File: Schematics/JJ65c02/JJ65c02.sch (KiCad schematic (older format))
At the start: 22 parts, among them U1 74HC00, U2 74HC02, X1 1Mhz

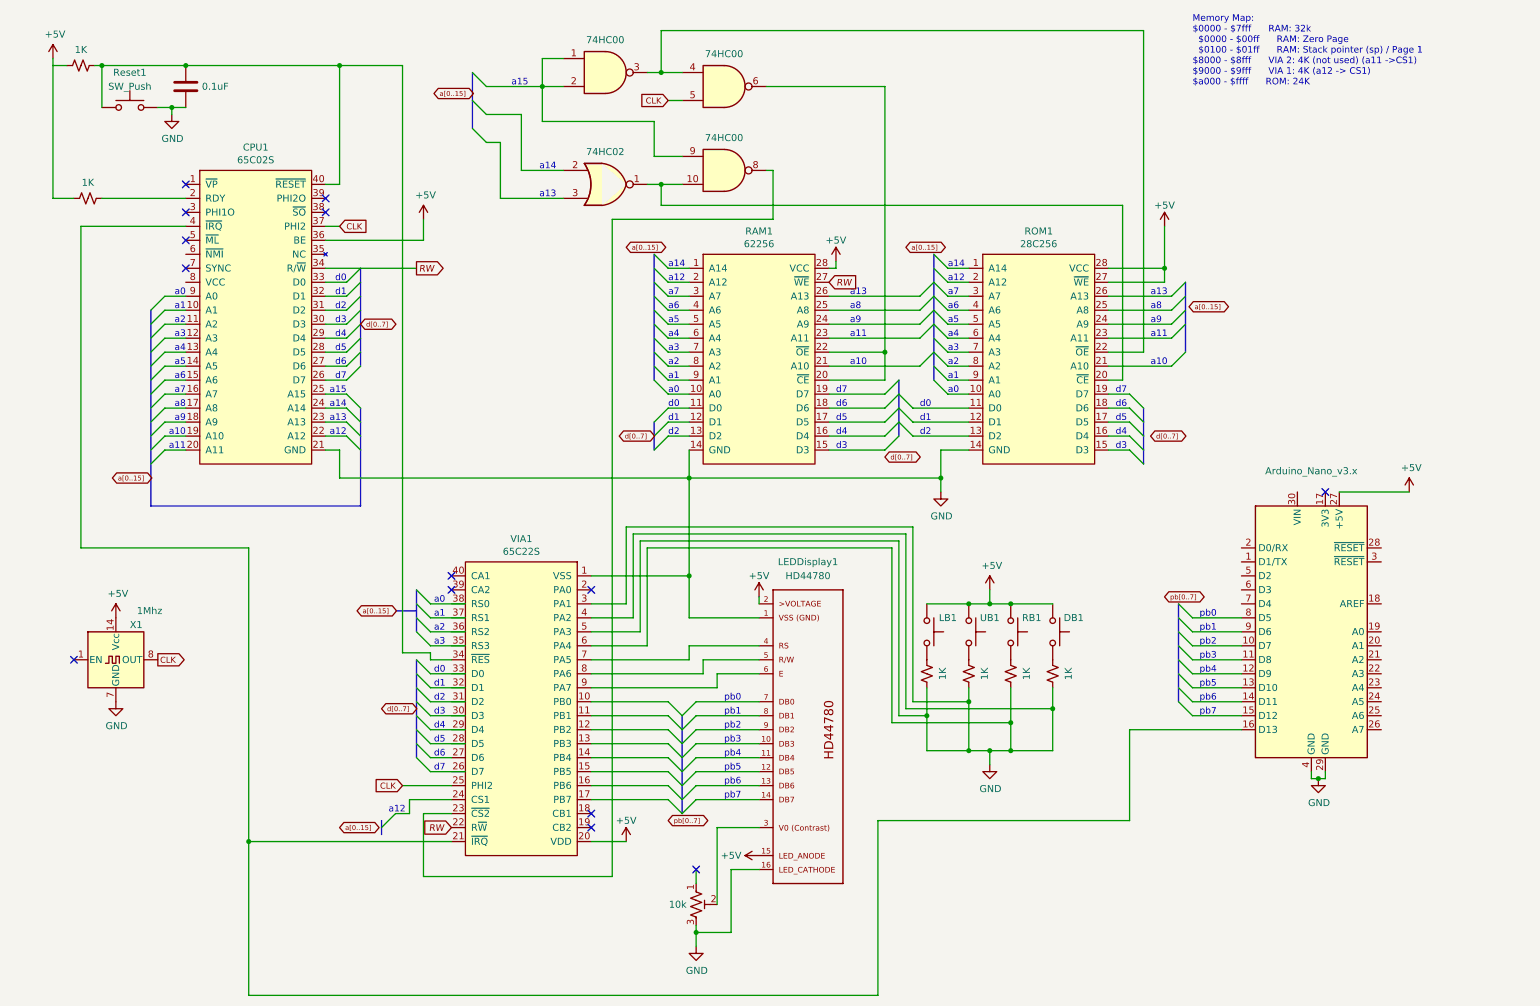
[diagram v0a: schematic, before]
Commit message: 6551 updates
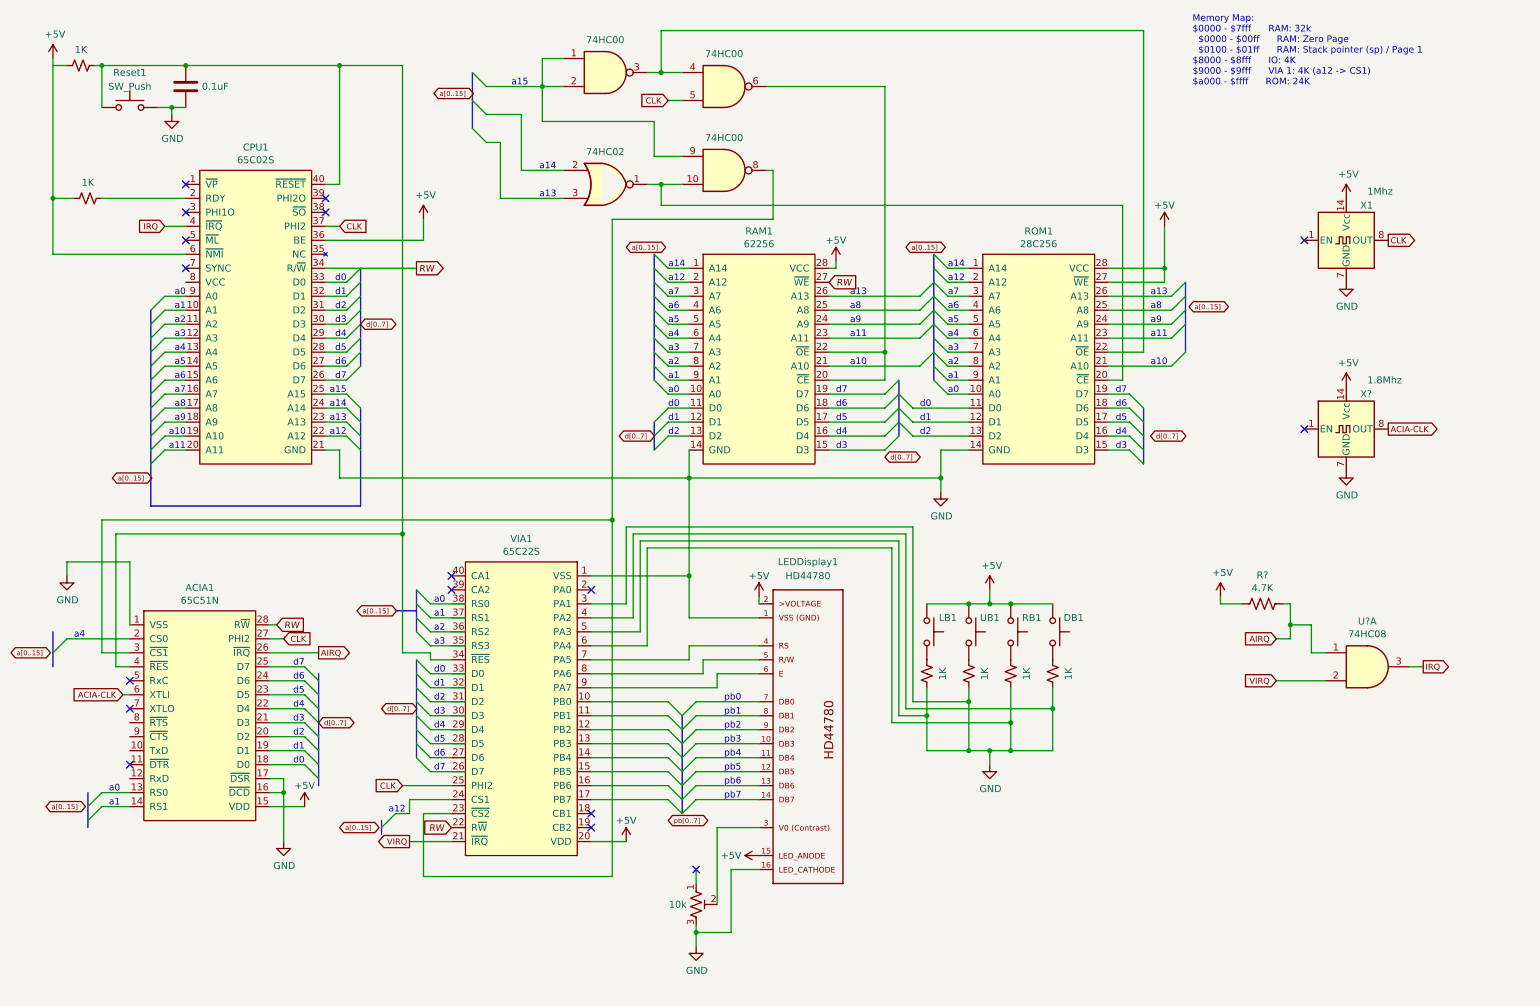
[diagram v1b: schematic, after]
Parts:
- removed A1: Arduino_Nano_v3.x, Module:Arduino_Nano, symbol MCU_Module:Arduino_Nano_v3.x
- added ACIA1: 65C51N, Package_DIP:DIP-28_W15.24mm_Socket, symbol 6502:65C51N
- added R?: 4.7K, symbol Device:R_US
- added U?: 74HC08, symbol 74xx:74LS08
- added X?: 1.8Mhz, Oscillator:Oscillator_DIP-14, symbol Oscillator:CXO_DIP14
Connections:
- net labels added: ACIA-CLK, AIRQ, IRQ, VIRQ
- wire segments 262 -> 284
- no-connect marks 14 -> 17
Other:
- note added: "Memory Map:\n$0000 - $7fff RAM: 32k\n $0000 - $00ff RAM: Zero Page\n $0100 - $01ff RAM: Stack pointer (sp) / Page 1\n$8000 - $8fff IO: 4K\n$9000 - $9fff VIA 1: 4K (a12 -> CS1)\n$a000 - $ffff ROM: 24K"
- note removed: "Memory Map:\n$0000 - $7fff RAM: 32k\n $0000 - $00ff RAM: Zero Page\n $0100 - $01ff RAM: Stack pointer (sp) / Page 1\n$8000 - $8fff VIA 2: 4K (not used) (a11 ->CS1)\n$9000 - $9fff VIA 1: 4K (a12 -> CS1)\n$a000 - $ffff ROM: 24K"
- moved on the sheet: X1
